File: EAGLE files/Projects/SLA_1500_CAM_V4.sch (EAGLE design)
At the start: 88 parts, among them J2 JST GH SM06B, J3 MOLEX 53261-03, J4 MOLEX 53261-04, J5 MOLEX 53261-04, J6 MOLEX 53261-04, U11 TXS0102, U2 TPS73633DCQR, U8 TXS0102, U9 TXS0102

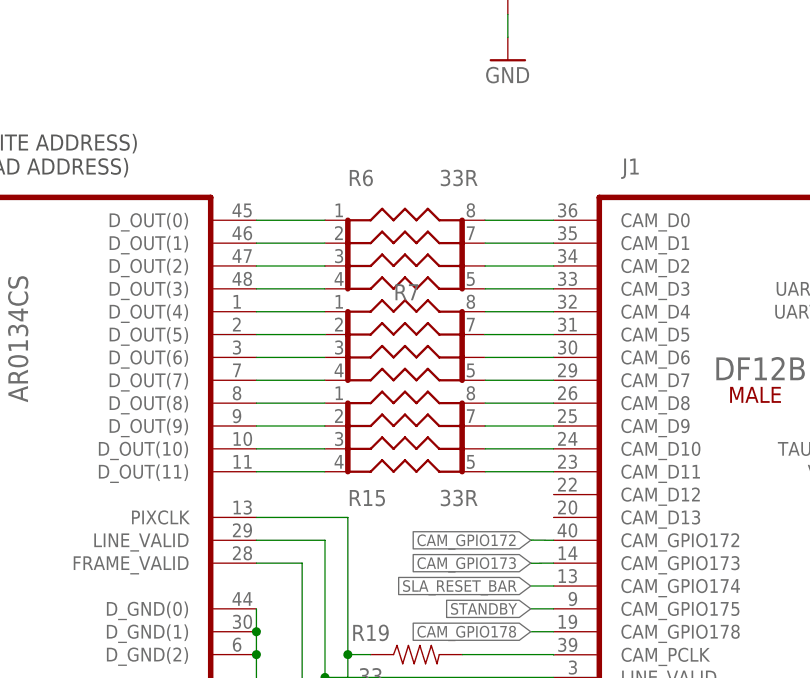
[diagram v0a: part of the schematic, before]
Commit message: Update SLA1500 CAM V4 .brd
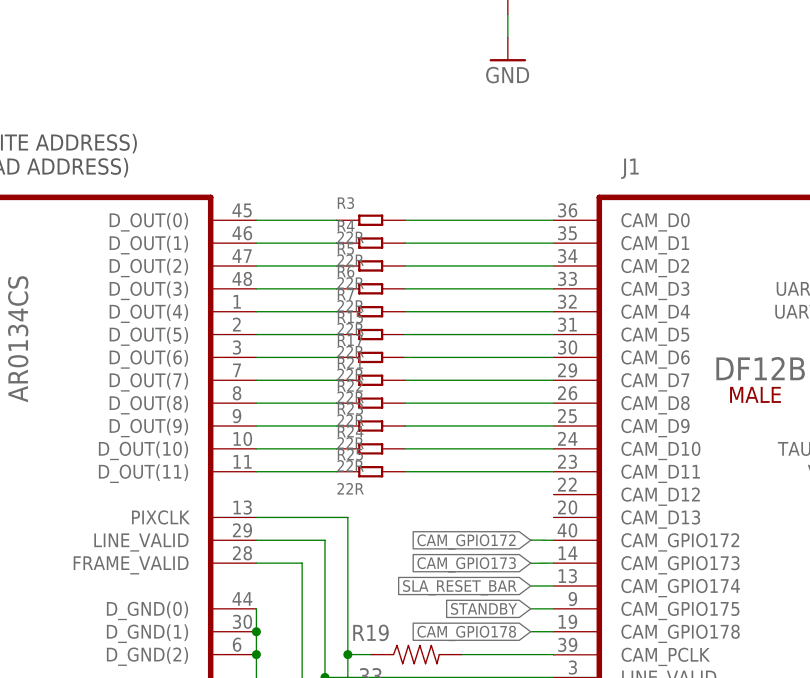
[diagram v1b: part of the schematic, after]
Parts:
- added R17, R21, R22, R23, R24, R25, R3, R4, R5: 22R, Seeed-Resistor:SMD-RES-22R-1%-1/16W(0402)
- R15, R6: value 33R -> 22R; device Sightline:YC124-JR-0733RL -> Seeed-Resistor:SMD-RES-22R-1%-1/16W(0402)
- R7: value (none) -> 22R; device Sightline:YC124-JR-0733RL -> Seeed-Resistor:SMD-RES-22R-1%-1/16W(0402)
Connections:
- removed net N$10 (its old number): R6.4, U1.D_OUT(3)
- removed net N$50: R15.4, U1.D_OUT(11)
- removed net N$51: J1.CAM_D11, R15.5
- new net N$12: R15.1, U1.D_OUT(5)
- new net N$2: R3.1, U1.D_OUT(0)
- new net N$3: J1.CAM_D0, R3.2
- net N$11: now also J1.CAM_D4, R7.2; no longer J1.CAM_D3, R6.5
- net N$14: now also J1.CAM_D5, R15.2; no longer J1.CAM_D4, R7.8
- net N$22: now also R17.1, U1.D_OUT(6); no longer R7.2, U1.D_OUT(5)
- net N$24: now also J1.CAM_D6, R17.2; no longer J1.CAM_D5, R7.7
- net N$4: now also R4.1, U1.D_OUT(1); no longer R6.1, U1.D_OUT(0)
- net N$40: now also R21.1, U1.D_OUT(7); no longer R7.3, U1.D_OUT(6)
- net N$41: now also J1.CAM_D7, R21.2; no longer J1.CAM_D6, R7.6
- net N$42: now also R22.1, U1.D_OUT(8); no longer R7.4, U1.D_OUT(7)
- net N$43: now also J1.CAM_D8, R22.2; no longer J1.CAM_D7, R7.5
- net N$44: now also R23.1, U1.D_OUT(9); no longer R15.1, U1.D_OUT(8)
- net N$45: now also J1.CAM_D9, R23.2; no longer J1.CAM_D8, R15.8
- net N$46: now also R24.1, U1.D_OUT(10); no longer R15.2, U1.D_OUT(9)
- net N$47: now also J1.CAM_D10, R24.2; no longer J1.CAM_D9, R15.7
- net N$48: now also R25.1, U1.D_OUT(11); no longer R15.3, U1.D_OUT(10)
- net N$49: now also J1.CAM_D11, R25.2; no longer J1.CAM_D10, R15.6
- net N$5: now also J1.CAM_D1, R4.2; no longer J1.CAM_D0, R6.8
- net N$6: now also R5.1, U1.D_OUT(2); no longer R6.2, U1.D_OUT(1)
- net N$7: now also J1.CAM_D2, R5.2; no longer J1.CAM_D1, R6.7
- net N$8: now also R6.1, U1.D_OUT(3); no longer R6.3, U1.D_OUT(2)
- net N$9: now also J1.CAM_D3, R6.2; no longer J1.CAM_D2, R6.6
